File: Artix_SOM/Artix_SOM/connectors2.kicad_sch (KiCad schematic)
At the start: 2 parts

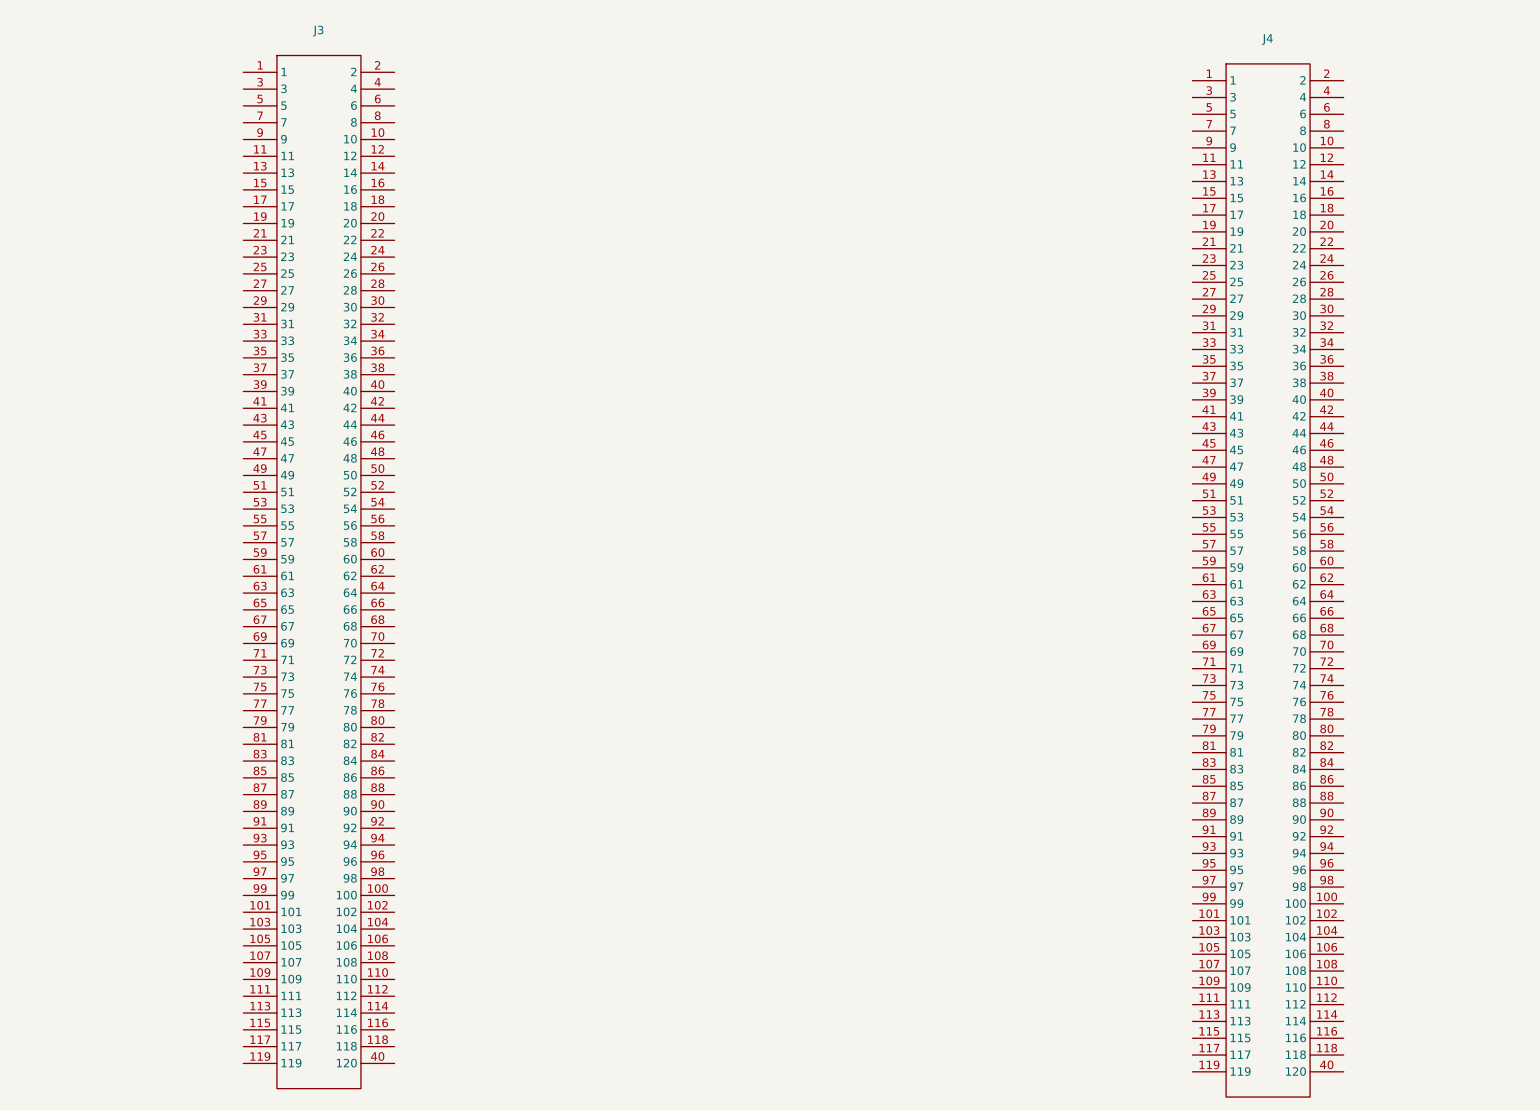
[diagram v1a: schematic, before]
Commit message: update
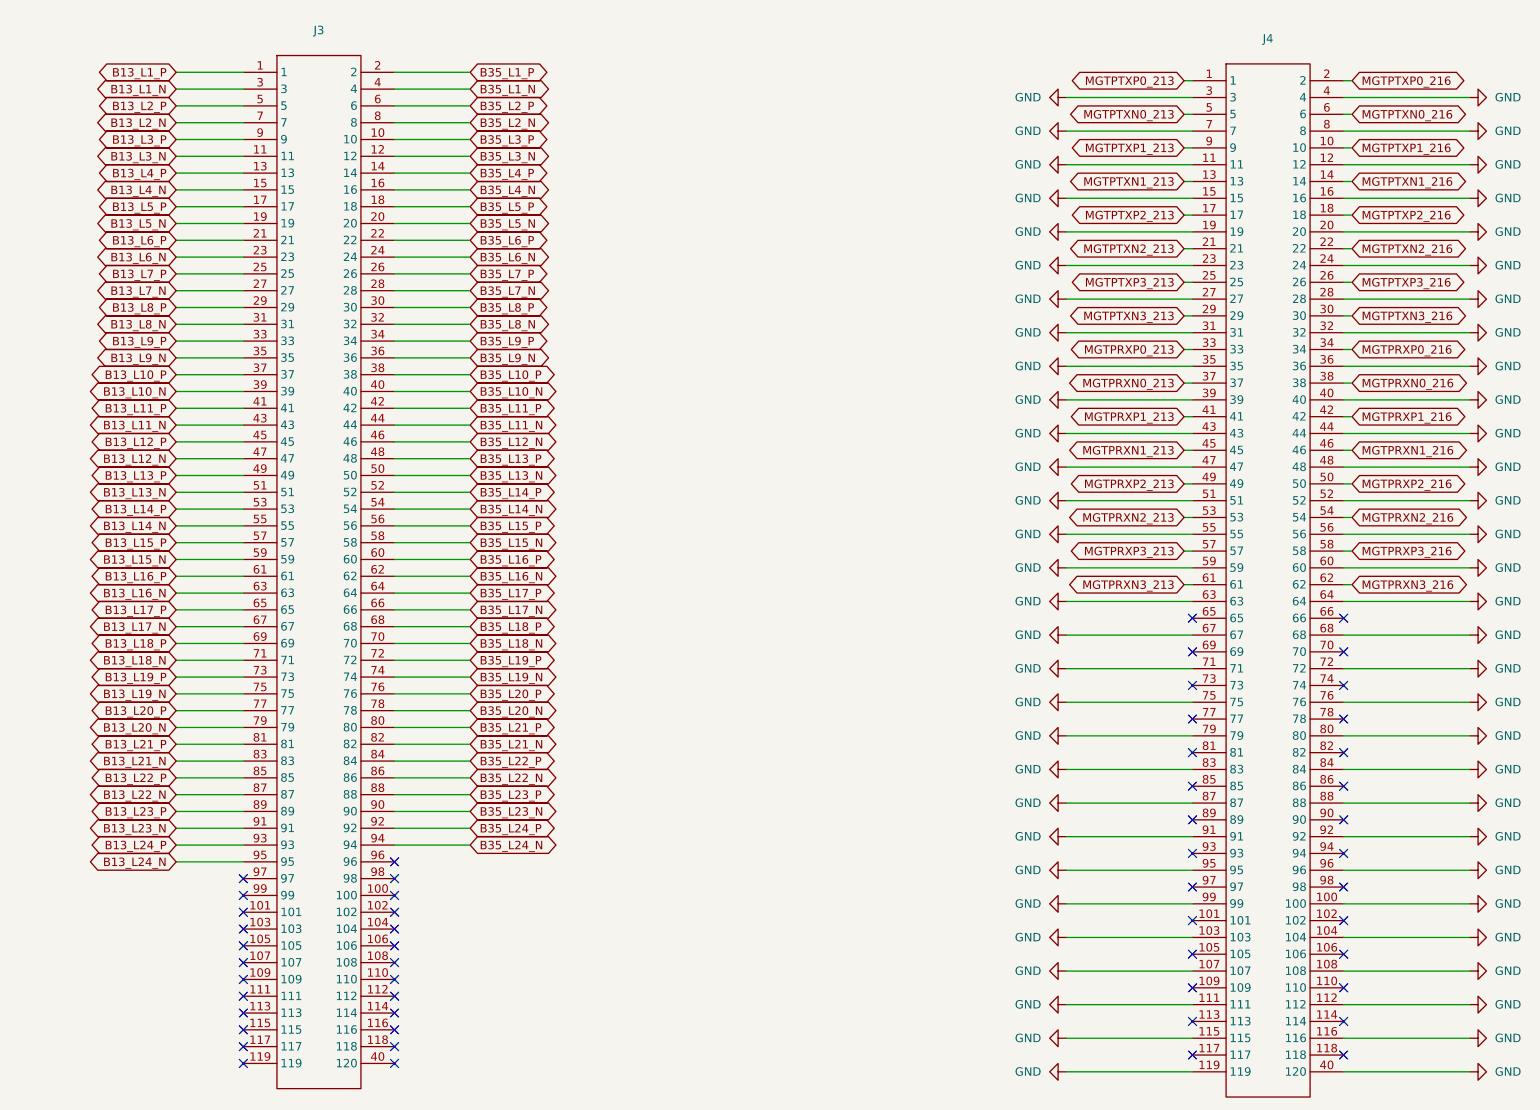
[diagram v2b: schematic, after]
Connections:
- net B13_L1_P: now reaches J3.1
- net B35_L3_P: now reaches J3.10
- net B13_L3_N: now reaches J3.11
- net B35_L3_N: now reaches J3.12
- net B13_L4_P: now reaches J3.13
- net B35_L4_P: now reaches J3.14
- net B13_L4_N: now reaches J3.15
- net B35_L4_N: now reaches J3.16
- net B13_L5_P: now reaches J3.17
- net B35_L5_P: now reaches J3.18
- net B13_L5_N: now reaches J3.19
- net B35_L1_P: now reaches J3.2
- net B35_L5_N: now reaches J3.20
- net B13_L6_P: now reaches J3.21
- net B35_L6_P: now reaches J3.22
- net B13_L6_N: now reaches J3.23
- net B35_L6_N: now reaches J3.24
- net B13_L7_P: now reaches J3.25
- net B35_L7_P: now reaches J3.26
- net B13_L7_N: now reaches J3.27
- net B35_L7_N: now reaches J3.28
- net B13_L8_P: now reaches J3.29
- net B13_L1_N: now reaches J3.3
- net B35_L8_P: now reaches J3.30
- net B13_L8_N: now reaches J3.31
- net B35_L8_N: now reaches J3.32
- net B13_L9_P: now reaches J3.33
- net B35_L9_P: now reaches J3.34
- net B13_L9_N: now reaches J3.35
- net B35_L9_N: now reaches J3.36
- net B13_L10_P: now reaches J3.37
- net B35_L10_P: now reaches J3.38
- net B13_L10_N: now reaches J3.39
- net B35_L1_N: now reaches J3.4
- net B35_L10_N: now reaches J3.40
- net B13_L11_P: now reaches J3.41
- net B35_L11_P: now reaches J3.42
- net B13_L11_N: now reaches J3.43
- net B35_L11_N: now reaches J3.44
- net B13_L12_P: now reaches J3.45
- net B35_L12_N: now reaches J3.46
- net B13_L12_N: now reaches J3.47
- net B35_L13_P: now reaches J3.48
- net B13_L13_P: now reaches J3.49
- net B13_L2_P: now reaches J3.5
- net B35_L13_N: now reaches J3.50
- net B13_L13_N: now reaches J3.51
- net B35_L14_P: now reaches J3.52
- net B13_L14_P: now reaches J3.53
- net B35_L14_N: now reaches J3.54
- net B13_L14_N: now reaches J3.55
- net B35_L15_P: now reaches J3.56
- net B13_L15_P: now reaches J3.57
- net B35_L15_N: now reaches J3.58
- net B13_L15_N: now reaches J3.59
- net B35_L2_P: now reaches J3.6
- net B35_L16_P: now reaches J3.60
- net B13_L16_P: now reaches J3.61
- net B35_L16_N: now reaches J3.62
- net B13_L16_N: now reaches J3.63
- net B35_L17_P: now reaches J3.64
- net B13_L17_P: now reaches J3.65
- net B35_L17_N: now reaches J3.66
- net B13_L17_N: now reaches J3.67
- net B35_L18_P: now reaches J3.68
- net B13_L18_P: now reaches J3.69
- net B13_L2_N: now reaches J3.7
- net B35_L18_N: now reaches J3.70
- net B13_L18_N: now reaches J3.71
- net B35_L19_P: now reaches J3.72
- net B13_L19_P: now reaches J3.73
- net B35_L19_N: now reaches J3.74
- net B13_L19_N: now reaches J3.75
- net B35_L20_P: now reaches J3.76
- net B13_L20_P: now reaches J3.77
- net B35_L20_N: now reaches J3.78
- net B13_L20_N: now reaches J3.79
- net B35_L2_N: now reaches J3.8
- net B35_L21_P: now reaches J3.80
- net B13_L21_P: now reaches J3.81
- net B35_L21_N: now reaches J3.82
- net B13_L21_N: now reaches J3.83
- net B35_L22_P: now reaches J3.84
- net B13_L22_P: now reaches J3.85
- net B35_L22_N: now reaches J3.86
- net B13_L22_N: now reaches J3.87
- net B35_L23_P: now reaches J3.88
- net B13_L23_P: now reaches J3.89
- net B13_L3_P: now reaches J3.9
- net B35_L23_N: now reaches J3.90
- net B13_L23_N: now reaches J3.91
- net B35_L24_P: now reaches J3.92
- net B13_L24_P: now reaches J3.93
- net B35_L24_N: now reaches J3.94
- net B13_L24_N: now reaches J3.95
- net MGTPTXP0_213: now reaches J4.1
- net MGTPTXP1_216: now reaches J4.10
- net GND: now reaches J4.100
- net GND: now also J4.103, J4.104, J4.107, J4.108, J4.11, J4.111, J4.112, J4.115, J4.116, J4.119, J4.12, J4.15, J4.16, J4.19, J4.20, J4.23, J4.24, J4.27, J4.28, J4.3, J4.31, J4.32, J4.35, J4.36, J4.39, J4.4, J4.40, J4.43, J4.44, J4.47, J4.48, J4.51, J4.52, J4.55, J4.56, J4.59, J4.60, J4.63, J4.64, J4.67, J4.68, J4.7, J4.71, J4.72, J4.75, J4.76, J4.79, J4.8, J4.80, J4.83, J4.84, J4.87, J4.88, J4.91, J4.92, J4.95, J4.96, J4.99
- net MGTPTXN1_213: now reaches J4.13
- net MGTPTXN1_216: now reaches J4.14
- net MGTPTXP2_213: now reaches J4.17
- net MGTPTXP2_216: now reaches J4.18
- net MGTPTXP0_216: now reaches J4.2
- net MGTPTXN2_213: now reaches J4.21
- net MGTPTXN2_216: now reaches J4.22
- net MGTPTXP3_213: now reaches J4.25
- net MGTPTXP3_216: now reaches J4.26
- net MGTPTXN3_213: now reaches J4.29
- net MGTPTXN3_216: now reaches J4.30
- net MGTPRXP0_213: now reaches J4.33
- net MGTPRXP0_216: now reaches J4.34
- net MGTPRXN0_213: now reaches J4.37
- net MGTPRXN0_216: now reaches J4.38
- net MGTPRXP1_213: now reaches J4.41
- net MGTPRXP1_216: now reaches J4.42
- net MGTPRXN1_213: now reaches J4.45
- net MGTPRXN1_216: now reaches J4.46
- net MGTPRXP2_213: now reaches J4.49
- net MGTPTXN0_213: now reaches J4.5
- net MGTPRXP2_216: now reaches J4.50
- net MGTPRXN2_213: now reaches J4.53
- net MGTPRXN2_216: now reaches J4.54
- net MGTPRXP3_213: now reaches J4.57
- net MGTPRXP3_216: now reaches J4.58
- net MGTPTXN0_216: now reaches J4.6
- net MGTPRXN3_213: now reaches J4.61
- net MGTPRXN3_216: now reaches J4.62
- net MGTPTXP1_213: now reaches J4.9
- no-connect marks 0 -> 53

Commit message: update
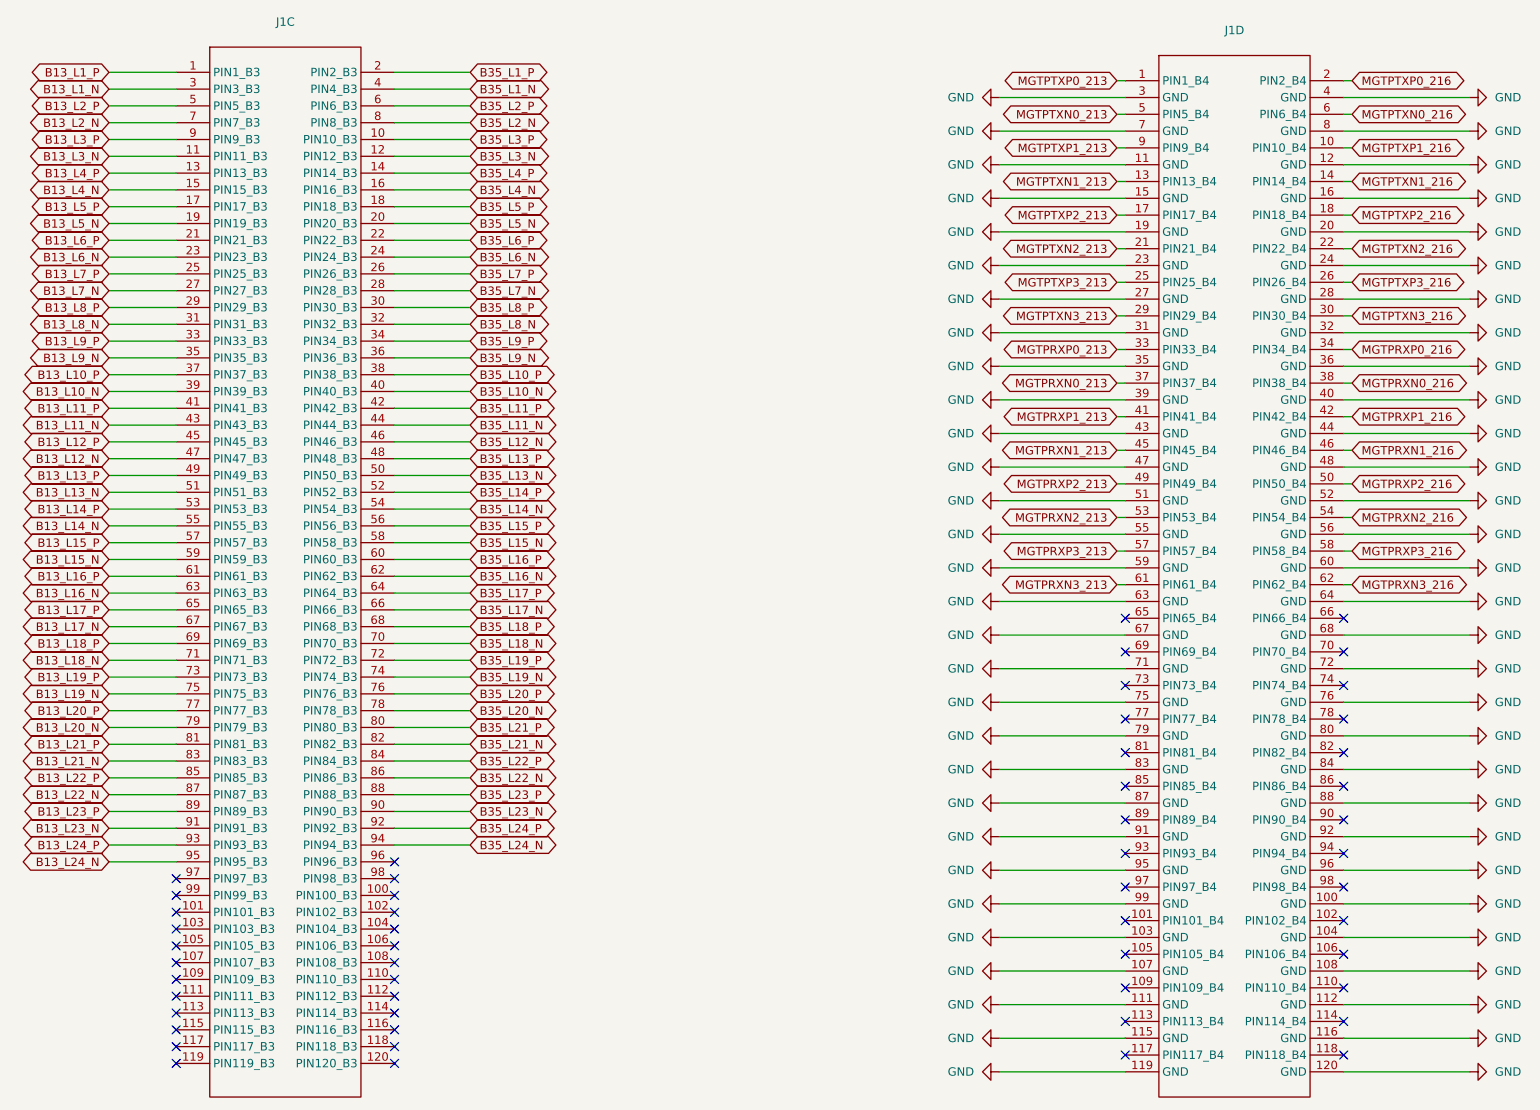
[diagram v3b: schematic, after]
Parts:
- removed J3, J4: ~, symbol Panasonic_connector:AXK6A2337YG
- added J1: ~, symbol SOM_library:SoM_male
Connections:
- net B13_L10_N: now also J1.39 (PIN39_B3)
- net B13_L10_P: now also J1.37 (PIN37_B3)
- net B13_L11_N: now also J1.43 (PIN43_B3)
- net B13_L11_P: now also J1.41 (PIN41_B3)
- net B13_L12_N: now also J1.47 (PIN47_B3)
- net B13_L12_P: now also J1.45 (PIN45_B3)
- net B13_L13_N: now also J1.51 (PIN51_B3)
- net B13_L13_P: now also J1.49 (PIN49_B3)
- net B13_L14_N: now also J1.55 (PIN55_B3)
- net B13_L14_P: now also J1.53 (PIN53_B3)
- net B13_L15_N: now also J1.59 (PIN59_B3)
- net B13_L15_P: now also J1.57 (PIN57_B3)
- net B13_L16_N: now also J1.63 (PIN63_B3)
- net B13_L16_P: now also J1.61 (PIN61_B3)
- net B13_L17_N: now also J1.67 (PIN67_B3)
- net B13_L17_P: now also J1.65 (PIN65_B3)
- net B13_L18_N: now also J1.71 (PIN71_B3)
- net B13_L18_P: now also J1.69 (PIN69_B3)
- net B13_L19_N: now also J1.75 (PIN75_B3)
- net B13_L19_P: now also J1.73 (PIN73_B3)
- net B13_L1_N: now also J1.3 (PIN3_B3)
- net B13_L1_P: now also J1.1 (PIN1_B3)
- net B13_L20_N: now also J1.79 (PIN79_B3)
- net B13_L20_P: now also J1.77 (PIN77_B3)
- net B13_L21_N: now also J1.83 (PIN83_B3)
- net B13_L21_P: now also J1.81 (PIN81_B3)
- net B13_L22_N: now also J1.87 (PIN87_B3)
- net B13_L22_P: now also J1.85 (PIN85_B3)
- net B13_L23_N: now also J1.91 (PIN91_B3)
- net B13_L23_P: now also J1.89 (PIN89_B3)
- net B13_L24_N: now also J1.95 (PIN95_B3)
- net B13_L24_P: now also J1.93 (PIN93_B3)
- net B13_L2_N: now also J1.7 (PIN7_B3)
- net B13_L2_P: now also J1.5 (PIN5_B3)
- net B13_L3_N: now also J1.11 (PIN11_B3)
- net B13_L3_P: now also J1.9 (PIN9_B3)
- net B13_L4_N: now also J1.15 (PIN15_B3)
- net B13_L4_P: now also J1.13 (PIN13_B3)
- net B13_L5_N: now also J1.19 (PIN19_B3)
- net B13_L5_P: now also J1.17 (PIN17_B3)
- net B13_L6_N: now also J1.23 (PIN23_B3)
- net B13_L6_P: now also J1.21 (PIN21_B3)
- net B13_L7_N: now also J1.27 (PIN27_B3)
- net B13_L7_P: now also J1.25 (PIN25_B3)
- net B13_L8_N: now also J1.31 (PIN31_B3)
- net B13_L8_P: now also J1.29 (PIN29_B3)
- net B13_L9_N: now also J1.35 (PIN35_B3)
- net B13_L9_P: now also J1.33 (PIN33_B3)
- net B35_L10_N: now also J1.40 (PIN40_B3)
- net B35_L10_P: now also J1.38 (PIN38_B3)
- net B35_L11_N: now also J1.44 (PIN44_B3)
- net B35_L11_P: now also J1.42 (PIN42_B3)
- net B35_L12_N: now also J1.46 (PIN46_B3)
- net B35_L13_N: now also J1.50 (PIN50_B3)
- net B35_L13_P: now also J1.48 (PIN48_B3)
- net B35_L14_N: now also J1.54 (PIN54_B3)
- net B35_L14_P: now also J1.52 (PIN52_B3)
- net B35_L15_N: now also J1.58 (PIN58_B3)
- net B35_L15_P: now also J1.56 (PIN56_B3)
- net B35_L16_N: now also J1.62 (PIN62_B3)
- net B35_L16_P: now also J1.60 (PIN60_B3)
- net B35_L17_N: now also J1.66 (PIN66_B3)
- net B35_L17_P: now also J1.64 (PIN64_B3)
- net B35_L18_N: now also J1.70 (PIN70_B3)
- net B35_L18_P: now also J1.68 (PIN68_B3)
- net B35_L19_N: now also J1.74 (PIN74_B3)
- net B35_L19_P: now also J1.72 (PIN72_B3)
- net B35_L1_N: now also J1.4 (PIN4_B3)
- net B35_L1_P: now also J1.2 (PIN2_B3)
- net B35_L20_N: now also J1.78 (PIN78_B3)
- net B35_L20_P: now also J1.76 (PIN76_B3)
- net B35_L21_N: now also J1.82 (PIN82_B3)
- net B35_L21_P: now also J1.80 (PIN80_B3)
- net B35_L22_N: now also J1.86 (PIN86_B3)
- net B35_L22_P: now also J1.84 (PIN84_B3)
- net B35_L23_N: now also J1.90 (PIN90_B3)
- net B35_L23_P: now also J1.88 (PIN88_B3)
- net B35_L24_N: now also J1.94 (PIN94_B3)
- net B35_L24_P: now also J1.92 (PIN92_B3)
- net B35_L2_N: now also J1.8 (PIN8_B3)
- net B35_L2_P: now also J1.6 (PIN6_B3)
- net B35_L3_N: now also J1.12 (PIN12_B3)
- net B35_L3_P: now also J1.10 (PIN10_B3)
- net B35_L4_N: now also J1.16 (PIN16_B3)
- net B35_L4_P: now also J1.14 (PIN14_B3)
- net B35_L5_N: now also J1.20 (PIN20_B3)
- net B35_L5_P: now also J1.18 (PIN18_B3)
- net B35_L6_N: now also J1.24 (PIN24_B3)
- net B35_L6_P: now also J1.22 (PIN22_B3)
- net B35_L7_N: now also J1.28 (PIN28_B3)
- net B35_L7_P: now also J1.26 (PIN26_B3)
- net B35_L8_N: now also J1.32 (PIN32_B3)
- net B35_L8_P: now also J1.30 (PIN30_B3)
- net B35_L9_N: now also J1.36 (PIN36_B3)
- net B35_L9_P: now also J1.34 (PIN34_B3)
- net GND: now also J1.100 (GND), J1.103 (GND), J1.104 (GND), J1.107 (GND), J1.108 (GND), J1.11 (GND), J1.111 (GND), J1.112 (GND), J1.115 (GND), J1.116 (GND), J1.119 (GND), J1.12 (GND), J1.120 (GND), J1.15 (GND), J1.16 (GND), J1.19 (GND), J1.20 (GND), J1.23 (GND), J1.24 (GND), J1.27 (GND), J1.28 (GND), J1.3 (GND), J1.31 (GND), J1.32 (GND), J1.35 (GND), J1.36 (GND), J1.39 (GND), J1.4 (GND), J1.40 (GND), J1.43 (GND), J1.44 (GND), J1.47 (GND), J1.48 (GND), J1.51 (GND), J1.52 (GND), J1.55 (GND), J1.56 (GND), J1.59 (GND), J1.60 (GND), J1.63 (GND), J1.64 (GND), J1.67 (GND), J1.68 (GND), J1.7 (GND), J1.71 (GND), J1.72 (GND), J1.75 (GND), J1.76 (GND), J1.79 (GND), J1.8 (GND), J1.80 (GND), J1.83 (GND), J1.84 (GND), J1.87 (GND), J1.88 (GND), J1.91 (GND), J1.92 (GND), J1.95 (GND), J1.96 (GND), J1.99 (GND)
- net MGTPRXN0_213: now also J1.37 (PIN37_B4)
- net MGTPRXN0_216: now also J1.38 (PIN38_B4)
- net MGTPRXN1_213: now also J1.45 (PIN45_B4)
- net MGTPRXN1_216: now also J1.46 (PIN46_B4)
- net MGTPRXN2_213: now also J1.53 (PIN53_B4)
- net MGTPRXN2_216: now also J1.54 (PIN54_B4)
- net MGTPRXN3_213: now also J1.61 (PIN61_B4)
- net MGTPRXN3_216: now also J1.62 (PIN62_B4)
- net MGTPRXP0_213: now also J1.33 (PIN33_B4)
- net MGTPRXP0_216: now also J1.34 (PIN34_B4)
- net MGTPRXP1_213: now also J1.41 (PIN41_B4)
- net MGTPRXP1_216: now also J1.42 (PIN42_B4)
- net MGTPRXP2_213: now also J1.49 (PIN49_B4)
- net MGTPRXP2_216: now also J1.50 (PIN50_B4)
- net MGTPRXP3_213: now also J1.57 (PIN57_B4)
- net MGTPRXP3_216: now also J1.58 (PIN58_B4)
- net MGTPTXN0_213: now also J1.5 (PIN5_B4)
- net MGTPTXN0_216: now also J1.6 (PIN6_B4)
- net MGTPTXN1_213: now also J1.13 (PIN13_B4)
- net MGTPTXN1_216: now also J1.14 (PIN14_B4)
- net MGTPTXN2_213: now also J1.21 (PIN21_B4)
- net MGTPTXN2_216: now also J1.22 (PIN22_B4)
- net MGTPTXN3_213: now also J1.29 (PIN29_B4)
- net MGTPTXN3_216: now also J1.30 (PIN30_B4)
- net MGTPTXP0_213: now also J1.1 (PIN1_B4)
- net MGTPTXP0_216: now also J1.2 (PIN2_B4)
- net MGTPTXP1_213: now also J1.9 (PIN9_B4)
- net MGTPTXP1_216: now also J1.10 (PIN10_B4)
- net MGTPTXP2_213: now also J1.17 (PIN17_B4)
- net MGTPTXP2_216: now also J1.18 (PIN18_B4)
- net MGTPTXP3_213: now also J1.25 (PIN25_B4)
- net MGTPTXP3_216: now also J1.26 (PIN26_B4)
